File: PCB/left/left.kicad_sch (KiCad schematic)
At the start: 2 parts, among them U1 COM-09032

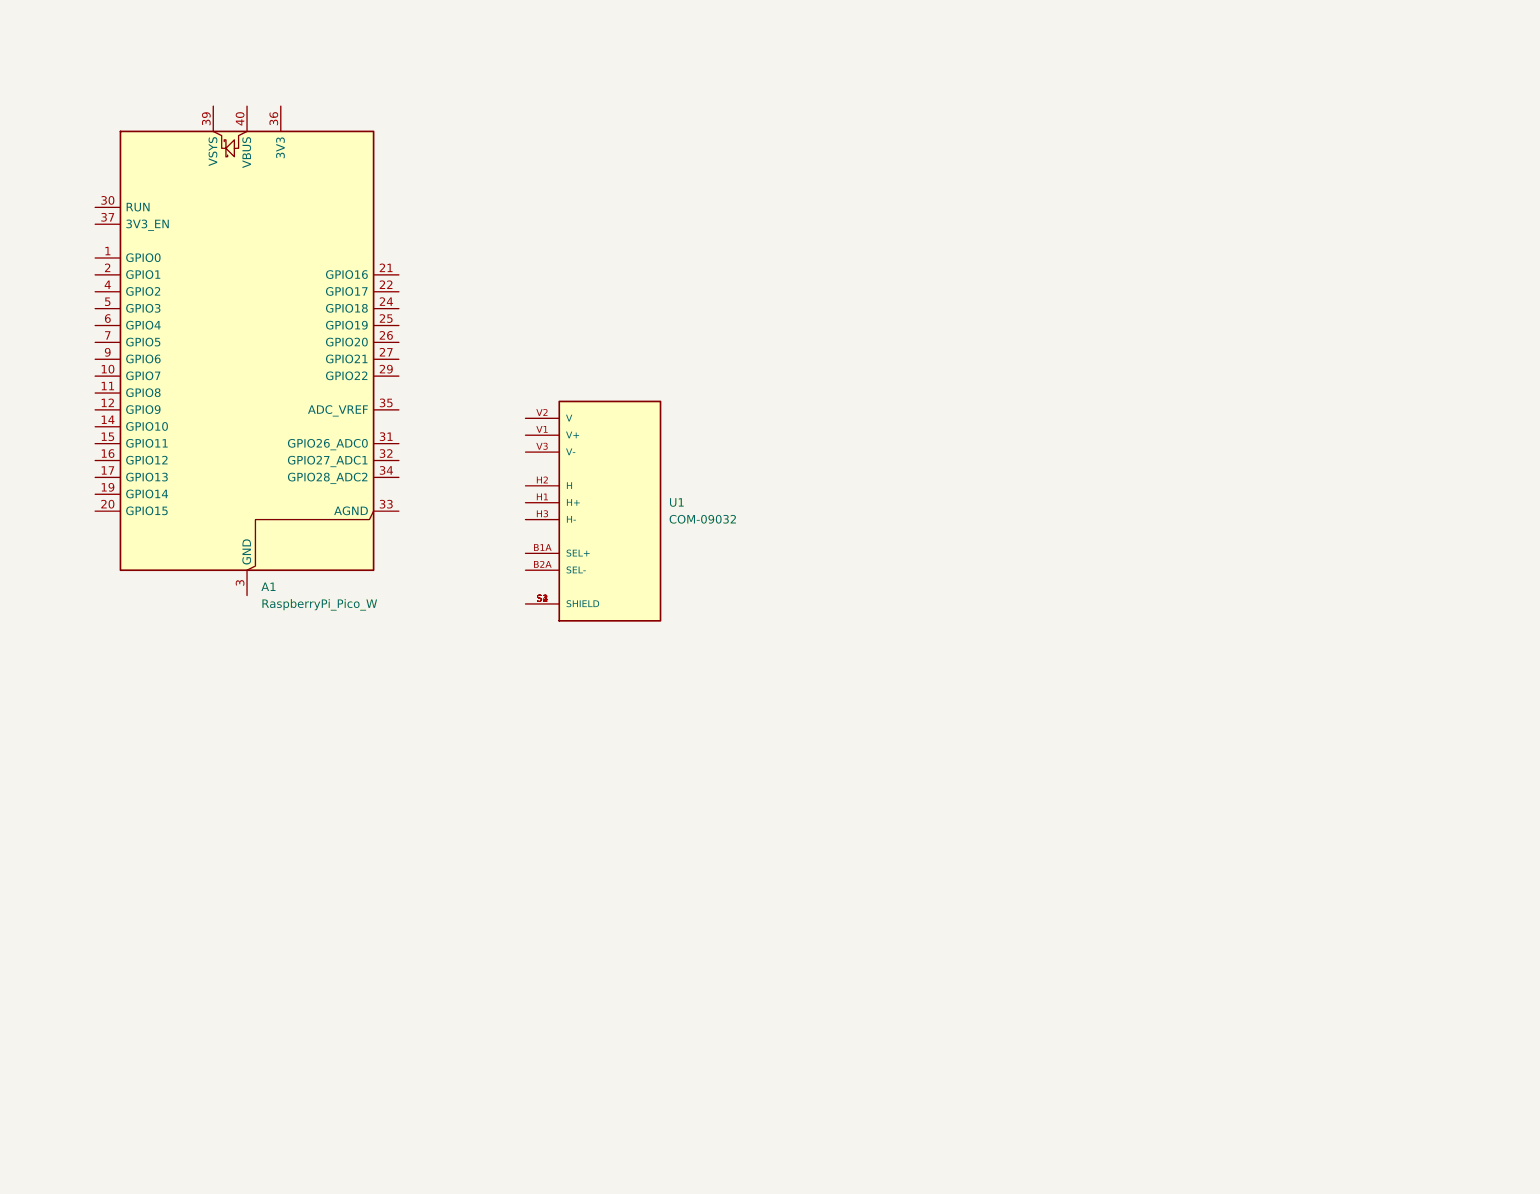
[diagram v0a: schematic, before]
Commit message: [ MAY 31 // GLOW ]
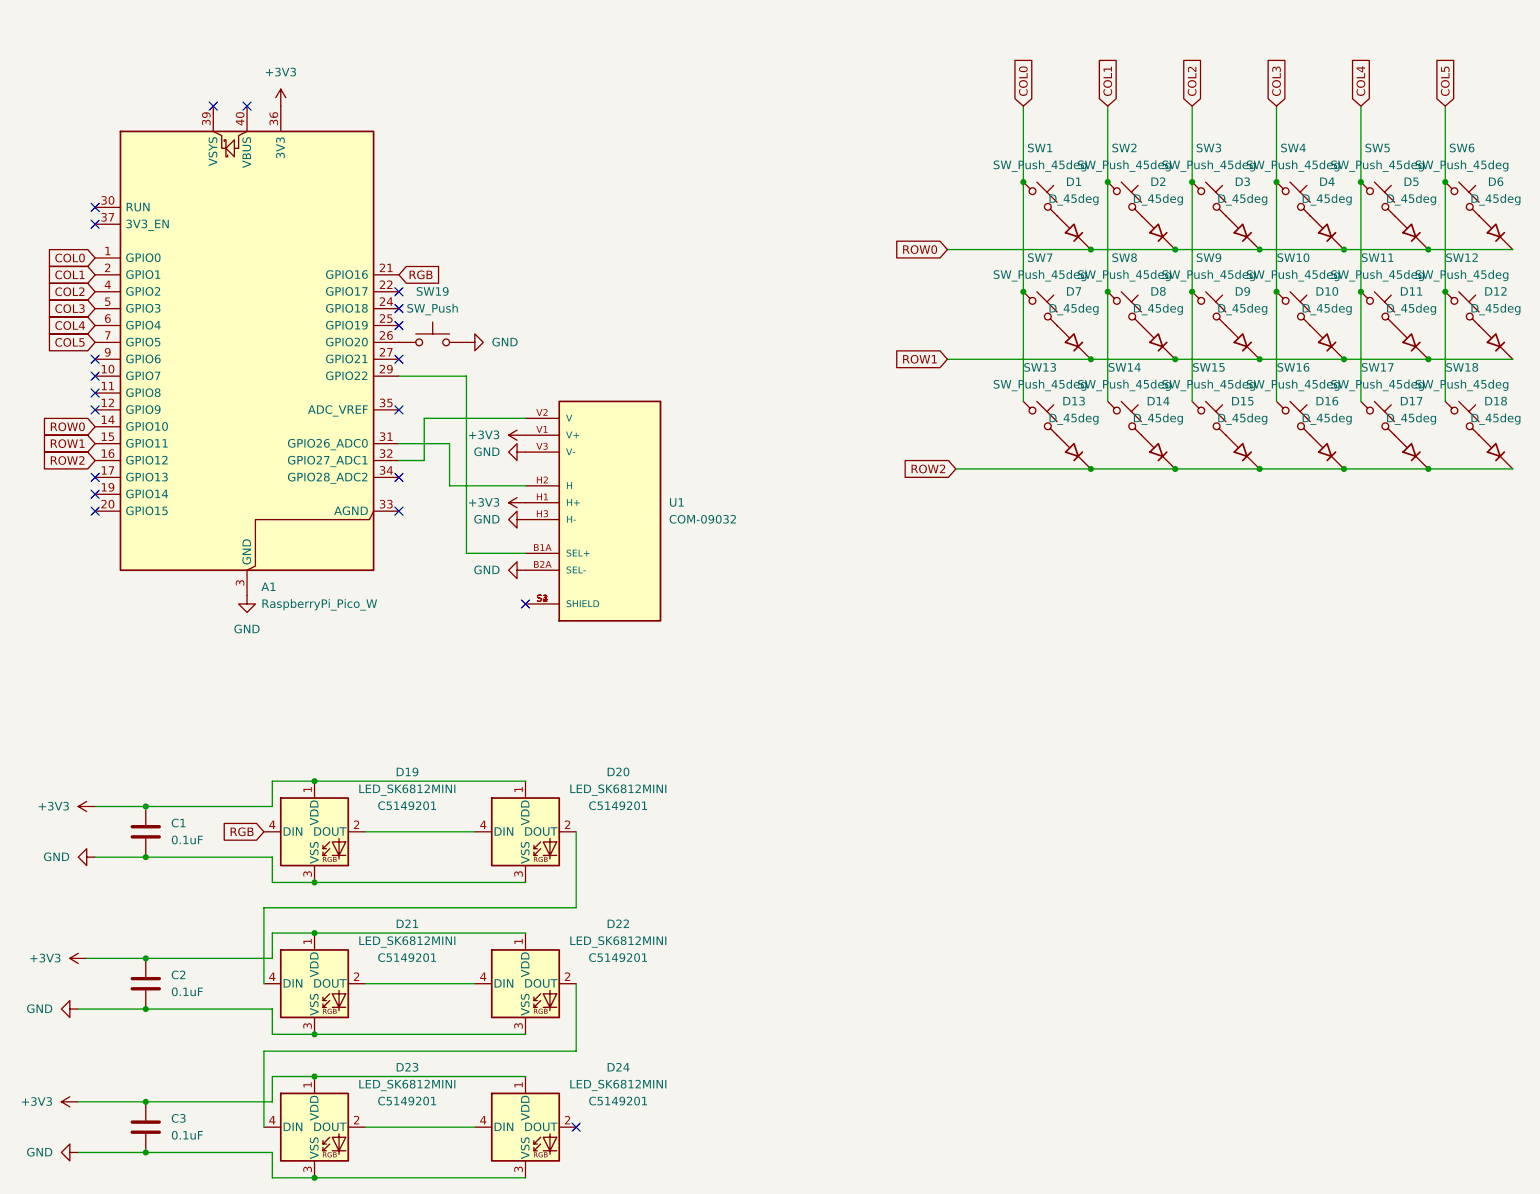
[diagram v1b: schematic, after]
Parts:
- added C1, C2, C3: 0.1uF, Capacitor_THT:C_Disc_D3.0mm_W1.6mm_P2.50mm, symbol Device:C
- added D1, D10, D11, D12, D13, D14, D15, D16, D17, D18, D2, D3, D4, D5, D6, D7, D8, D9: D_45deg, Diode_THT:D_DO-35_SOD27_P7.62mm_Horizontal, symbol Device:D_45deg
- added D19, D20, D21, D22, D23, D24: LED_SK6812MINI, ScottoKeebs_Components:LED_SK6812MINI, symbol ScottoKeebs:LED_SK6812MINI
- added SW1, SW10, SW11, SW12, SW13, SW14, SW15, SW16, SW17, SW18, SW2, SW3, SW4, SW5, SW6, SW7, SW8, SW9: SW_Push_45deg, ScottoKeebs_Hotswap:Hotswap_MX_Plated, symbol Switch:SW_Push_45deg
- added SW19: SW_Push, ScottoKeebs_Hotswap:Hotswap_MX_Plated, symbol Switch:SW_Push
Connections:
- net COL0: now reaches A1.1 (GPIO0)
- net COL0: now also SW1.1, SW13.1, SW7.1
- net GND: now reaches A1.13 (GND), A1.18 (GND), A1.23 (GND), A1.28 (GND), A1.3 (GND), A1.38 (GND), A1.8 (GND)
- net GND: now also U1.B2A (SEL-), U1.H3 (H-), U1.V3 (V-), C1.2, C2.2, C3.2, D19.3 (VSS), D20.3 (VSS), D21.3 (VSS), D22.3 (VSS), D23.3 (VSS), D24.3 (VSS), SW19.2
- net ROW0: now reaches A1.14 (GPIO10)
- net ROW0: now also D1.1 (K), D2.1 (K), D3.1 (K), D4.1 (K), D5.1 (K), D6.1 (K)
- net ROW1: now reaches A1.15 (GPIO11)
- net ROW1: now also D10.1 (K), D11.1 (K), D12.1 (K), D7.1 (K), D8.1 (K), D9.1 (K)
- net ROW2: now reaches A1.16 (GPIO12)
- net ROW2: now also D13.1 (K), D14.1 (K), D15.1 (K), D16.1 (K), D17.1 (K), D18.1 (K)
- net COL1: now reaches A1.2 (GPIO1)
- net COL1: now also SW14.1, SW2.1, SW8.1
- net RGB: now reaches A1.21 (GPIO16)
- net RGB: now also D19.4 (DIN)
- net at A1.26 (GPIO20): now also SW19.1
- net at A1.29 (GPIO22): now also U1.B1A (SEL+)
- net at A1.31 (GPIO26_ADC0): now also U1.H2 (H)
- net at A1.32 (GPIO27_ADC1): now also U1.V2 (V)
- net +3V3: now reaches A1.36 (3V3)
- net +3V3: now also U1.H1 (H+), U1.V1 (V+), C1.1, C2.1, C3.1, D19.1 (VDD), D20.1 (VDD), D21.1 (VDD), D22.1 (VDD), D23.1 (VDD), D24.1 (VDD)
- net COL2: now reaches A1.4 (GPIO2)
- net COL2: now also SW15.1, SW3.1, SW9.1
- net COL3: now reaches A1.5 (GPIO3)
- net COL3: now also SW10.1, SW16.1, SW4.1
- net COL4: now reaches A1.6 (GPIO4)
- net COL4: now also SW11.1, SW17.1, SW5.1
- net COL5: now reaches A1.7 (GPIO5)
- net COL5: now also SW12.1, SW18.1, SW6.1
- new net: D5.2 (A), SW5.2
- new net: D21.2 (DOUT), D22.4 (DIN)
- new net: D20.2 (DOUT), D21.4 (DIN)
- new net: D15.2 (A), SW15.2
- new net: D14.2 (A), SW14.2
- new net: D22.2 (DOUT), D23.4 (DIN)
- new net: D2.2 (A), SW2.2
- new net: D9.2 (A), SW9.2
- new net: D10.2 (A), SW10.2
- new net: D11.2 (A), SW11.2
- new net: D1.2 (A), SW1.2
- new net: D19.2 (DOUT), D20.4 (DIN)
- new net: D16.2 (A), SW16.2
- new net: D23.2 (DOUT), D24.4 (DIN)
- new net: D3.2 (A), SW3.2
- new net: D4.2 (A), SW4.2
- new net: D8.2 (A), SW8.2
- new net: D13.2 (A), SW13.2
- new net: D7.2 (A), SW7.2
- new net: D6.2 (A), SW6.2
- new net: D12.2 (A), SW12.2
- new net: D18.2 (A), SW18.2
- new net: D17.2 (A), SW17.2
- no-connect marks 0 -> 20

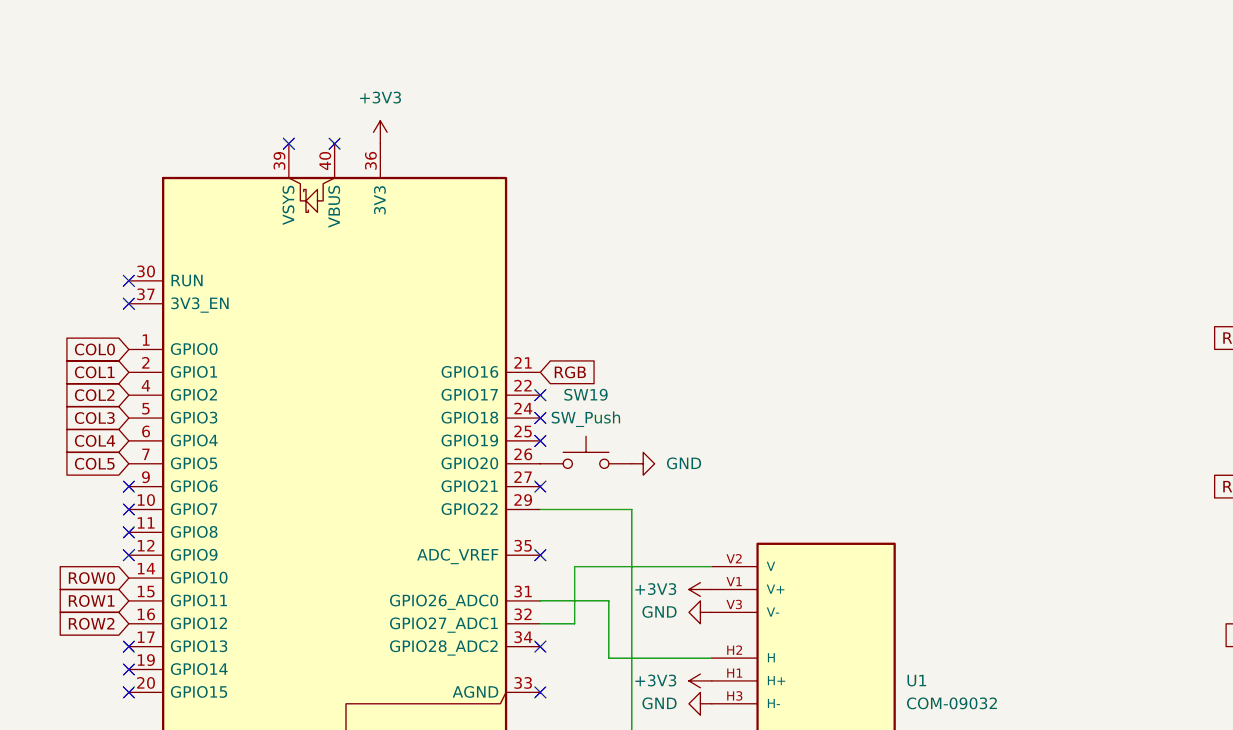
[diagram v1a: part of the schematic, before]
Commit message: [ JUN 4 // ARRANGEMENTS ]
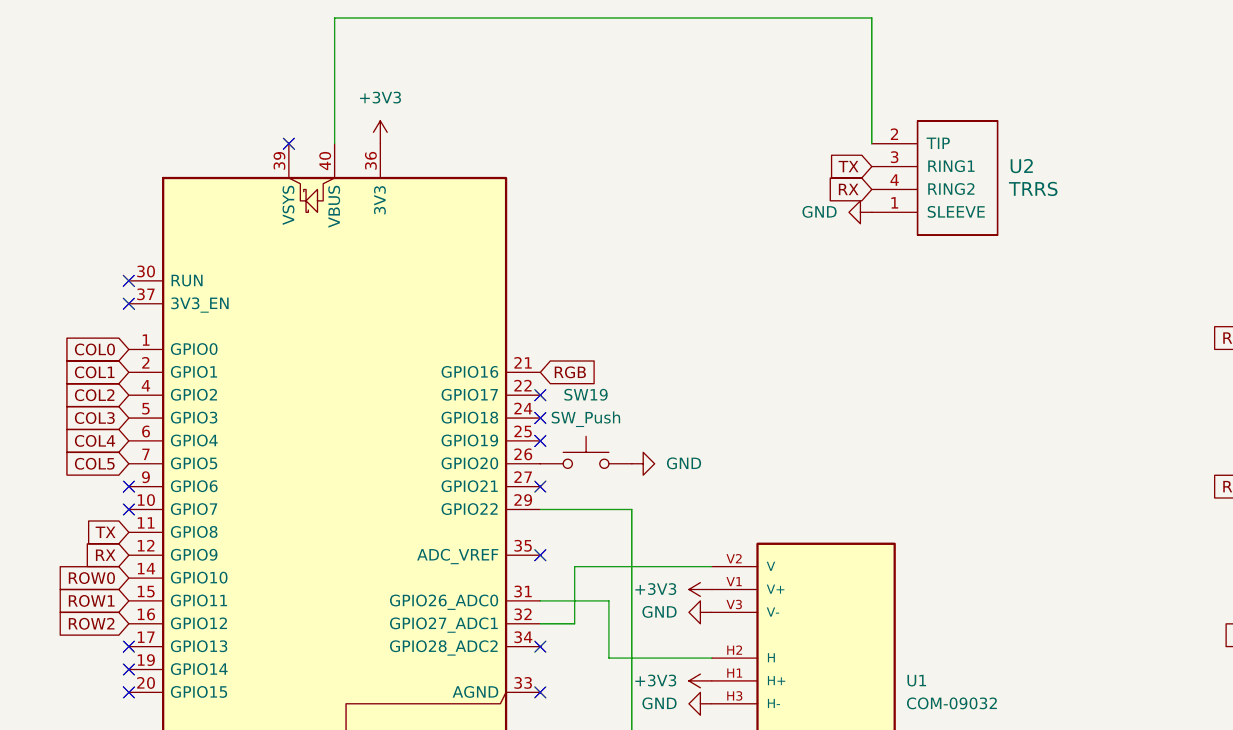
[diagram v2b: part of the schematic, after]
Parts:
- added U2: TRRS, ScottoKeebs_Components:TRRS_PJ-320A, symbol ScottoKeebs:Placeholder_TRRS
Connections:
- net GND: now also U2.1 (SLEEVE)
- net TX: now reaches A1.11 (GPIO8)
- net TX: now also U2.3 (RING1)
- net RX: now reaches A1.12 (GPIO9)
- net RX: now also U2.4 (RING2)
- net at A1.40 (VBUS): now also U2.2 (TIP)
- no-connect marks 20 -> 17
